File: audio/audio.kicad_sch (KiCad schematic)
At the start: 0 parts

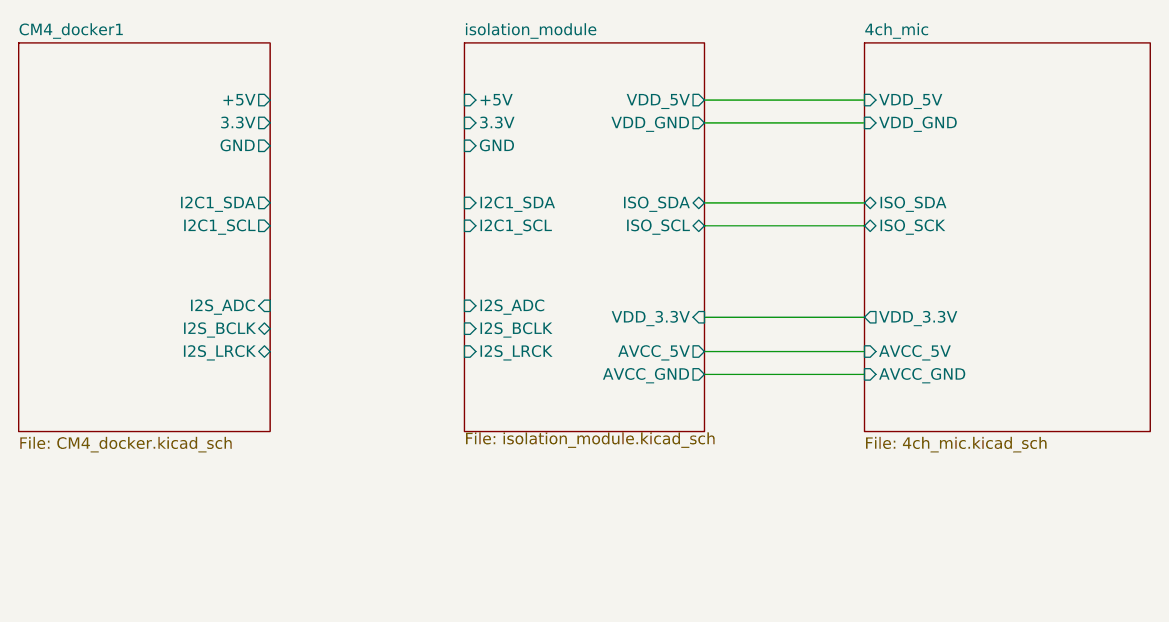
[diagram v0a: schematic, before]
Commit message: .
.
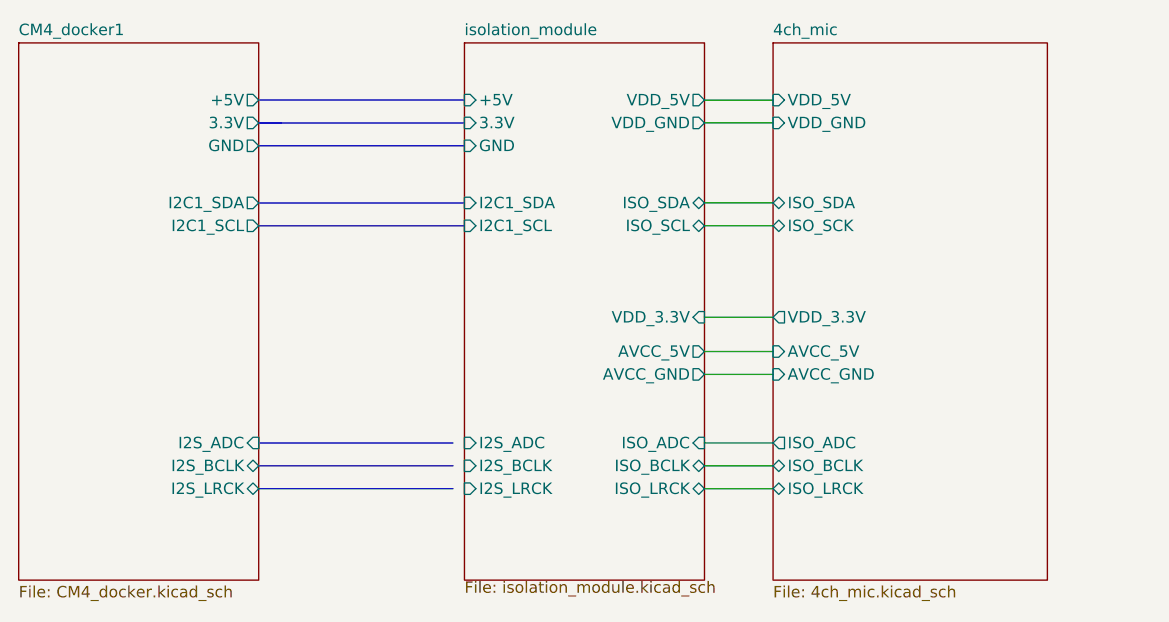
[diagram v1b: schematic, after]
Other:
- sheet 4ch_mic ports: added ISO_ADC, ISO_BCLK, ISO_LRCK; removed none
- sheet isolation_module ports: added ISO_ADC, ISO_BCLK, ISO_LRCK; removed none
